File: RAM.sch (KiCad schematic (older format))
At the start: 169 parts, among them J2 JTAG_01x06, J3 Conn_01x03_Male, U10 W25Q128JVS, U11 TPS62823DLC, U12 TPS62823DLC, U13 TPS62823DLC, U14 TPS62823DLC, U15 TPS62823DLC, U16 TPS62823DLC, U2 XC7K160T-FFG676, U3 IS43TR16512B-125KBLI, U4 IS43TR16512B-125KBLI, U5 TPS51200DRC, U6 KSZ9031RNXCA, U7 TUSB1310ZAY, U8 TC358778XBG, U9 SiI9022A, Y1 ABM8G-25.000MHZ-18-D2Y-T, Y2 ABM8G-20.000MHZ-18-D2Y-T

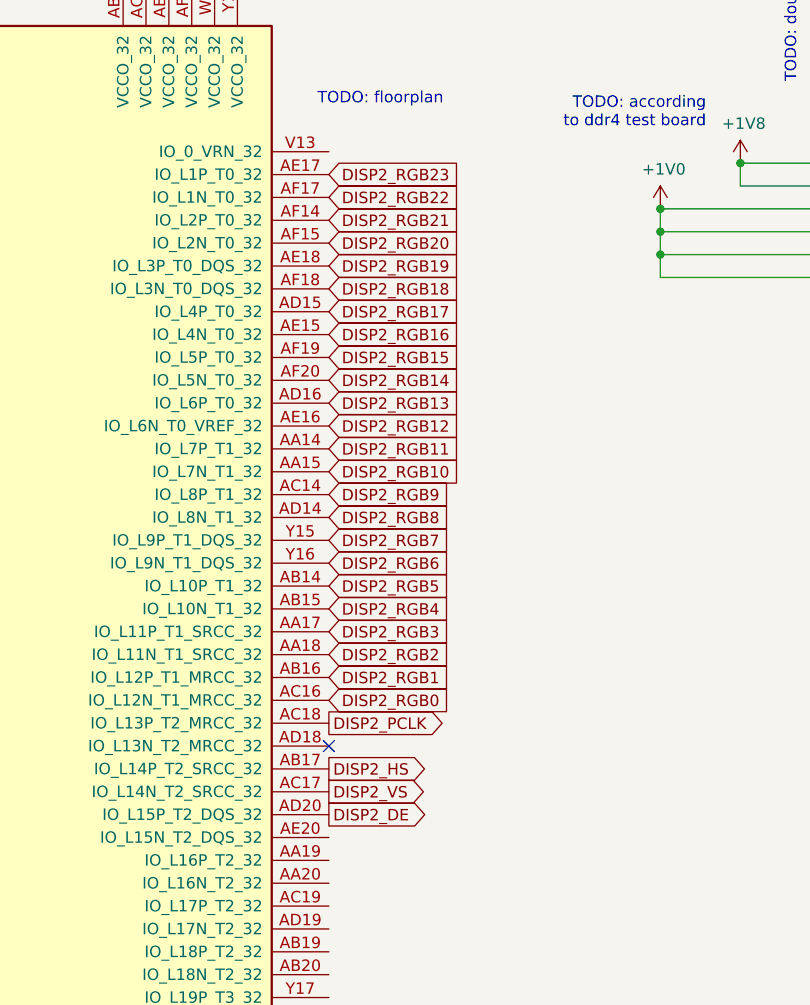
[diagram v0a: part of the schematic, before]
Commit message: DSI and some USB routing
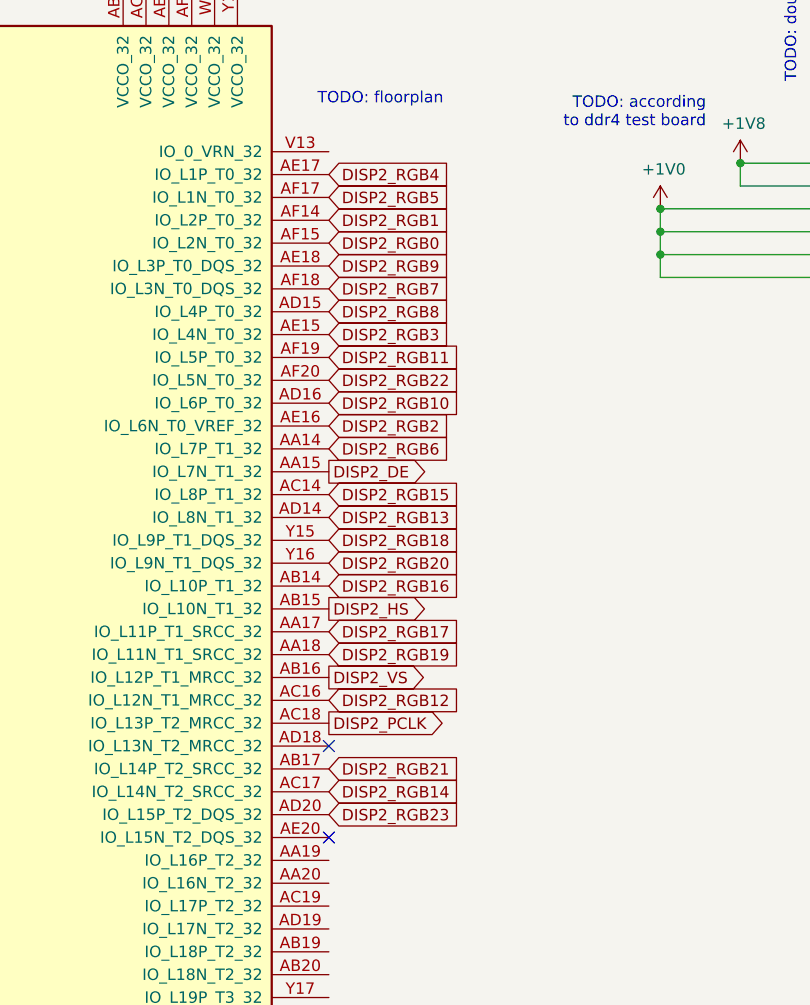
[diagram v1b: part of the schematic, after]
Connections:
- net DISP2_DE: now also U2.AA15 (IO_L7N_T1_32); no longer U2.AD20 (IO_L15P_T2_DQS_32)
- net DISP2_HS: now also U2.AB15 (IO_L10N_T1_32); no longer U2.AB17 (IO_L14P_T2_SRCC_32)
- net DISP2_RGB0: now also U2.AF15 (IO_L2N_T0_32); no longer U2.AC16 (IO_L12N_T1_MRCC_32)
- net DISP2_RGB1: now also U2.AF14 (IO_L2P_T0_32); no longer U2.AB16 (IO_L12P_T1_MRCC_32)
- net DISP2_RGB10: now also U2.AD16 (IO_L6P_T0_32); no longer U2.AA15 (IO_L7N_T1_32)
- net DISP2_RGB11: now also U2.AF19 (IO_L5P_T0_32); no longer U2.AA14 (IO_L7P_T1_32)
- net DISP2_RGB12: now also U2.AC16 (IO_L12N_T1_MRCC_32); no longer U2.AE16 (IO_L6N_T0_VREF_32)
- net DISP2_RGB13: now also U2.AD14 (IO_L8N_T1_32); no longer U2.AD16 (IO_L6P_T0_32)
- net DISP2_RGB14: now also U2.AC17 (IO_L14N_T2_SRCC_32); no longer U2.AF20 (IO_L5N_T0_32)
- net DISP2_RGB15: now also U2.AC14 (IO_L8P_T1_32); no longer U2.AF19 (IO_L5P_T0_32)
- net DISP2_RGB16: now also U2.AB14 (IO_L10P_T1_32); no longer U2.AE15 (IO_L4N_T0_32)
- net DISP2_RGB17: now also U2.AA17 (IO_L11P_T1_SRCC_32); no longer U2.AD15 (IO_L4P_T0_32)
- net DISP2_RGB18: now also U2.Y15 (IO_L9P_T1_DQS_32); no longer U2.AF18 (IO_L3N_T0_DQS_32)
- net DISP2_RGB19: now also U2.AA18 (IO_L11N_T1_SRCC_32); no longer U2.AE18 (IO_L3P_T0_DQS_32)
- net DISP2_RGB2: now also U2.AE16 (IO_L6N_T0_VREF_32); no longer U2.AA18 (IO_L11N_T1_SRCC_32)
- net DISP2_RGB20: now also U2.Y16 (IO_L9N_T1_DQS_32); no longer U2.AF15 (IO_L2N_T0_32)
- net DISP2_RGB21: now also U2.AB17 (IO_L14P_T2_SRCC_32); no longer U2.AF14 (IO_L2P_T0_32)
- net DISP2_RGB22: now also U2.AF20 (IO_L5N_T0_32); no longer U2.AF17 (IO_L1N_T0_32)
- net DISP2_RGB23: now also U2.AD20 (IO_L15P_T2_DQS_32); no longer U2.AE17 (IO_L1P_T0_32)
- net DISP2_RGB3: now also U2.AE15 (IO_L4N_T0_32); no longer U2.AA17 (IO_L11P_T1_SRCC_32)
- net DISP2_RGB4: now also U2.AE17 (IO_L1P_T0_32); no longer U2.AB15 (IO_L10N_T1_32)
- net DISP2_RGB5: now also U2.AF17 (IO_L1N_T0_32); no longer U2.AB14 (IO_L10P_T1_32)
- net DISP2_RGB6: now also U2.AA14 (IO_L7P_T1_32); no longer U2.Y16 (IO_L9N_T1_DQS_32)
- net DISP2_RGB7: now also U2.AF18 (IO_L3N_T0_DQS_32); no longer U2.Y15 (IO_L9P_T1_DQS_32)
- net DISP2_RGB8: now also U2.AD15 (IO_L4P_T0_32); no longer U2.AD14 (IO_L8N_T1_32)
- net DISP2_RGB9: now also U2.AE18 (IO_L3P_T0_DQS_32); no longer U2.AC14 (IO_L8P_T1_32)
- net DISP2_VS: now also U2.AB16 (IO_L12P_T1_MRCC_32); no longer U2.AC17 (IO_L14N_T2_SRCC_32)
- no-connect marks 22 -> 23
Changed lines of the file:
@@
 Text GLabel 12800 5000 0    50   Output ~ 0
 DISP1_DE
-Text GLabel 16800 4500 2    50   Input ~ 0
+Text GLabel 16800 2500 2    50   Input ~ 0
 DISP2_RGB0
-Text GLabel 16800 4400 2    50   Input ~ 0
+Text GLabel 16800 2400 2    50   Input ~ 0
 DISP2_RGB1
-Text GLabel 16800 4300 2    50   Input ~ 0
+Text GLabel 16800 3300 2    50   Input ~ 0
 DISP2_RGB2
-Text GLabel 16800 4200 2    50   Input ~ 0
+Text GLabel 16800 2900 2    50   Input ~ 0
 DISP2_RGB3
-Text GLabel 16800 4100 2    50   Input ~ 0
+Text GLabel 16800 2200 2    50   Input ~ 0
 DISP2_RGB4
-Text GLabel 16800 4000 2    50   Input ~ 0
+Text GLabel 16800 2300 2    50   Input ~ 0
 DISP2_RGB5
-Text GLabel 16800 3900 2    50   Input ~ 0
+Text GLabel 16800 3400 2    50   Input ~ 0
 DISP2_RGB6
-Text GLabel 16800 3800 2    50   Input ~ 0
+Text GLabel 16800 2700 2    50   Input ~ 0
 DISP2_RGB7
-Text GLabel 16800 3700 2    50   Input ~ 0
+Text GLabel 16800 2800 2    50   Input ~ 0
 DISP2_RGB8
-Text GLabel 16800 3600 2    50   Input ~ 0
-DISP2_RGB9
-Text GLabel 16800 3500 2    50   Input ~ 0
+Text GLabel 16800 3200 2    50   Input ~ 0
 DISP2_RGB10
-Text GLabel 16800 3400 2    50   Input ~ 0
+Text GLabel 16800 3000 2    50   Input ~ 0
 DISP2_RGB11
-Text GLabel 16800 3300 2    50   Input ~ 0
+Text GLabel 16800 4500 2    50   Input ~ 0
 DISP2_RGB12
-Text GLabel 16800 3200 2    50   Input ~ 0
+Text GLabel 16800 3700 2    50   Input ~ 0
 DISP2_RGB13
-Text GLabel 16800 3100 2    50   Input ~ 0
+Text GLabel 16800 4900 2    50   Input ~ 0
 DISP2_RGB14
-Text GLabel 16800 3000 2    50   Input ~ 0
+Text GLabel 16800 3600 2    50   Input ~ 0
 DISP2_RGB15
-Text GLabel 16800 2900 2    50   Input ~ 0
+Text GLabel 16800 4000 2    50   Input ~ 0
 DISP2_RGB16
-Text GLabel 16800 2800 2    50   Input ~ 0
+Text GLabel 16800 4200 2    50   Input ~ 0
 DISP2_RGB17
-Text GLabel 16800 2700 2    50   Input ~ 0
-DISP2_RGB18
-Text GLabel 16800 2600 2    50   Input ~ 0
+Text GLabel 16800 4300 2    50   Input ~ 0
 DISP2_RGB19
-Text GLabel 16800 2500 2    50   Input ~ 0
+Text GLabel 16800 3900 2    50   Input ~ 0
 DISP2_RGB20
-Text GLabel 16800 2400 2    50   Input ~ 0
+Text GLabel 16800 4800 2    50   Input ~ 0
 DISP2_RGB21
-Text GLabel 16800 2300 2    50   Input ~ 0
+Text GLabel 16800 3100 2    50   Input ~ 0
 DISP2_RGB22
-Text GLabel 16800 2200 2    50   Input ~ 0
+Text GLabel 16800 5000 2    50   Input ~ 0
 DISP2_RGB23
-Text GLabel 16800 4900 2    50   Output ~ 0
+Text GLabel 16800 4400 2    50   Output ~ 0
 DISP2_VS
-Text GLabel 16800 4800 2    50   Output ~ 0
+Text GLabel 16800 4100 2    50   Output ~ 0
 DISP2_HS
-Text GLabel 16800 5000 2    50   Output ~ 0
+Text GLabel 16800 3500 2    50   Output ~ 0
 DISP2_DE
 Text GLabel 17750 11650 2    50   Input ~ 0
@@
 Wire Wire Line
 	11000 13650 10900 13650
+NoConn ~ 16800 5100
+Text GLabel 16800 2600 2    50   Input ~ 0
+DISP2_RGB9
+Text GLabel 16800 3800 2    50   Input ~ 0
+DISP2_RGB18
 $EndSCHEMATC
